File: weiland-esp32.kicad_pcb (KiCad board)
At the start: 2 copper layers, 68.7 x 21.8 mm, 40 parts, among them CN1 SM05B-SRSS-TB (LF)(SN), CN2 SM04B-SRSS-TB (LF)(SN), CN3 SM04B-SRSS-TB (LF)(SN), CN4 SM02B-SRSS-TB (LF)(SN), CN5 SM02B-SRSS-TB (LF)(SN), U1 ESP32-WROOM-32E(8MB), U2 AMS1117-3.3_C347222, U3 MAX98357AETE_T, U5 ULN2003F12FN-7, U6 DZ127S-22-06-55

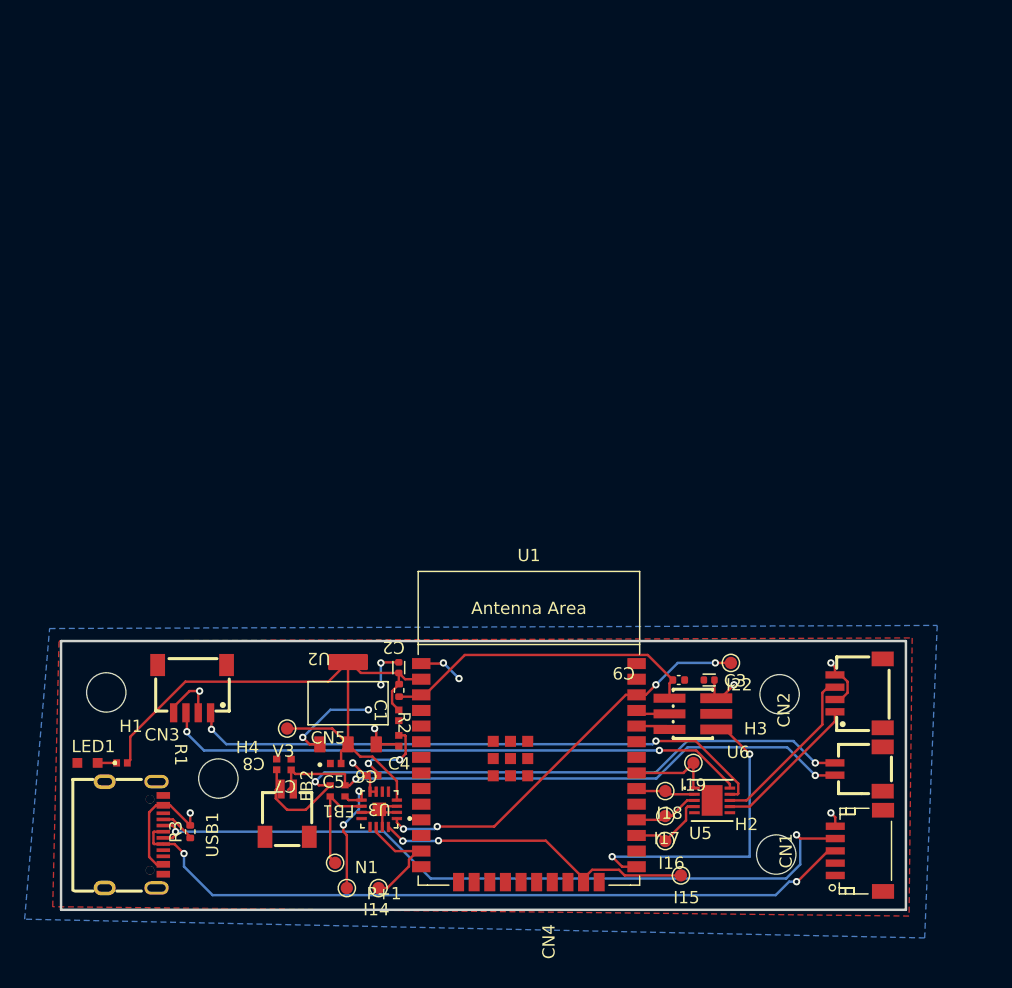
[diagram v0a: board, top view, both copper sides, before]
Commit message: fully routed board
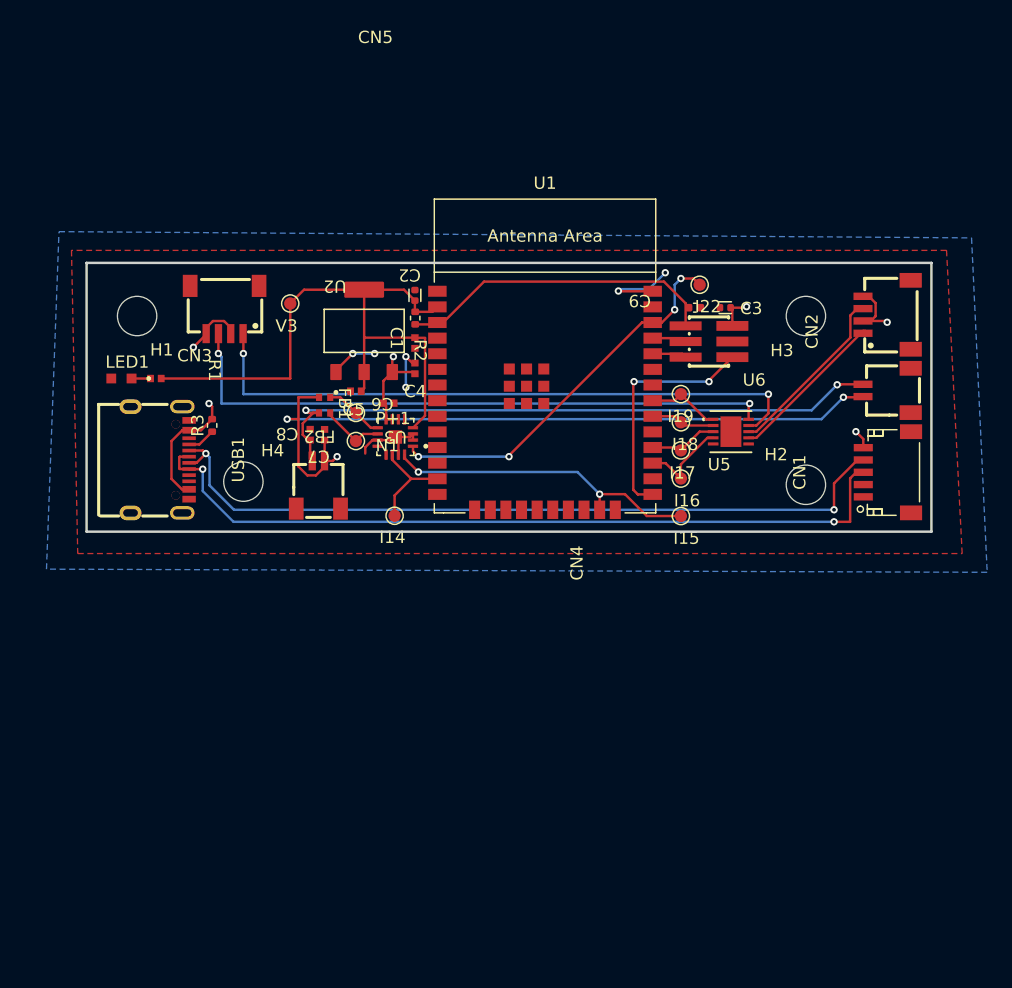
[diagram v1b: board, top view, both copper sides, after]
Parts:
- moved P+1 38.6 mm to (154.7, 35.3)
- moved V3 34.5 mm to (149.4, 26.4)
- moved N1 34.3 mm to (154.7, 37.6)
- moved R3 33.1 mm to (143.0, 36.3)
- moved FB1 32.0 mm to (152.1, 34.0), turned to 180 degrees
- moved LED1 31.4 mm to (135.6, 32.5)
- moved R1 31.4 mm to (138.4, 32.5)
- moved CN3 30.9 mm to (144.0, 26.9)
- moved CN1 30.9 mm to (197.9, 40.1)
- moved CN2 30.9 mm to (197.8, 27.3)
- moved CN4 30.9 mm to (197.8, 33.5)
- moved I22 30.8 mm to (182.6, 24.9)
- moved H3 30.8 mm to (191.3, 27.4)
- moved FB2 30.7 mm to (152.1, 35.3), turned to 180 degrees
- moved H1 30.7 mm to (136.9, 27.4)
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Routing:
- net /OUTP: track 49.2 -> 61.8 mm, vias 2 -> 3
- net GND: track 27.4 -> 21.4 mm, vias 8 -> 6
- net /IO0: track 25.4 -> 19.4 mm
- net /PRE-OUTP: track 10.8 -> 4.89 mm, vias 2 -> 0
- net /OUTB: track 47.9 -> 51.2 mm
- net /PRE-OUTN: track 8.44 -> 5.16 mm
- net /Dp: track 61.0 -> 63.9 mm
- net /OUTA: track 47.9 -> 50.0 mm
- net /IO22: track 33.3 -> 31.3 mm
- net +5V: track 31.2 -> 33.1 mm, vias 7 -> 6
- net +3.3V: track 53.2 -> 51.5 mm
- net /IO14: track 9.76 -> 8.29 mm
- net /Dn: track 61.4 -> 62.7 mm
- net /OUTN: track 53.7 -> 52.5 mm
- net /OUTD: track 12.2 -> 13.3 mm
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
